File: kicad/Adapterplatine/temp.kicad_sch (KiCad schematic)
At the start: 12 parts, among them X20 Conn_01x02_Pin, X22 Conn_01x02_Pin, X23 Conn_01x02_Pin, X56 Conn_01x02_Pin

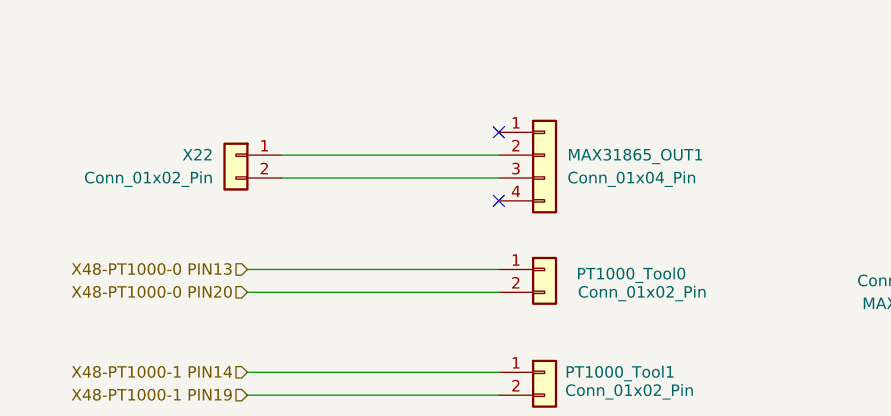
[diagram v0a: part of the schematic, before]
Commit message: Adapterplatine Version 1.0
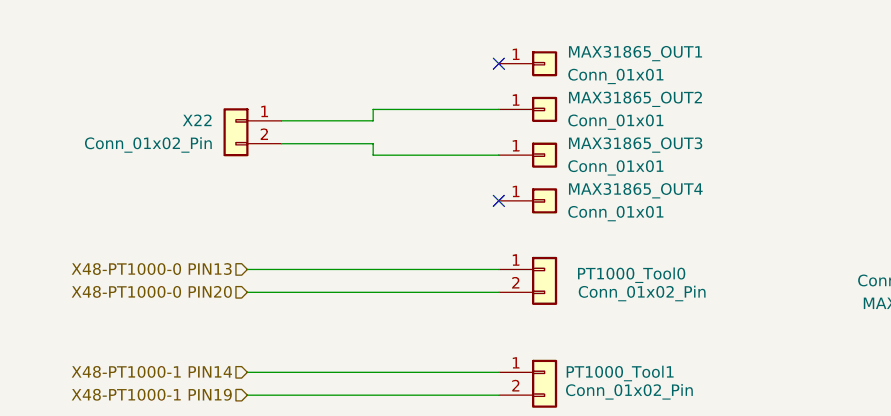
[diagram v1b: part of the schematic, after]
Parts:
- removed MAX31865_OUT1: Conn_01x04_Pin, TerminalBlock_Phoenix:TerminalBlock_Phoenix_PT-1,5-4-3.5-H_1x04_P3.50mm_Horizontal, symbol Connector_Generic:Conn_01x04
- added MAX31865_OUT1, MAX31865_OUT2, MAX31865_OUT3, MAX31865_OUT4: Conn_01x01, Connector_PinSocket_2.54mm:PinSocket_1x01_P2.54mm_Vertical, symbol Connector_Generic:Conn_01x01
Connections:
- net at X22.1 (Pin_1): now also MAX31865_OUT2.1 (Pin_1)
- net at X22.2 (Pin_2): now also MAX31865_OUT3.1 (Pin_1)
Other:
- moved on the sheet: X22
